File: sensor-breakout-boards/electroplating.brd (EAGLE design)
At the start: 25.4 x 25.4 mm, 4 parts, among them X1 Type-A Receptacle, X2 10-PIN-CONNECTOR

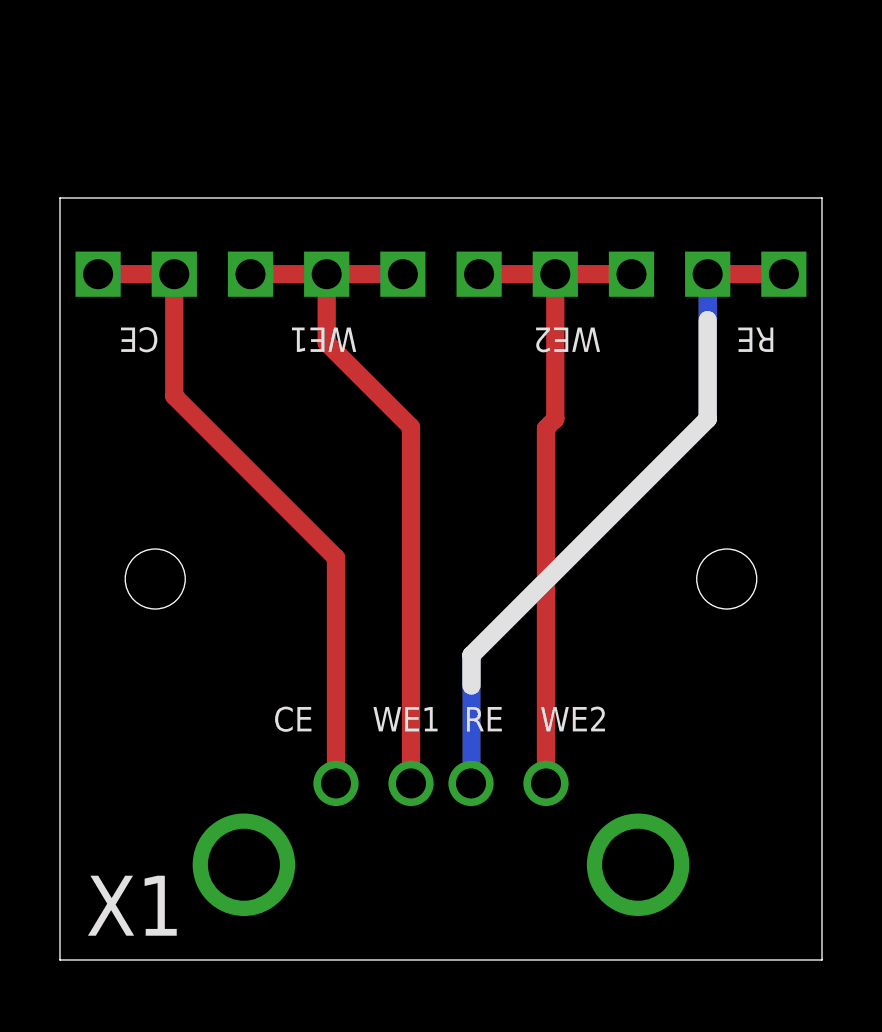
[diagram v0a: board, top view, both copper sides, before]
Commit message: made changes discussed at meeting
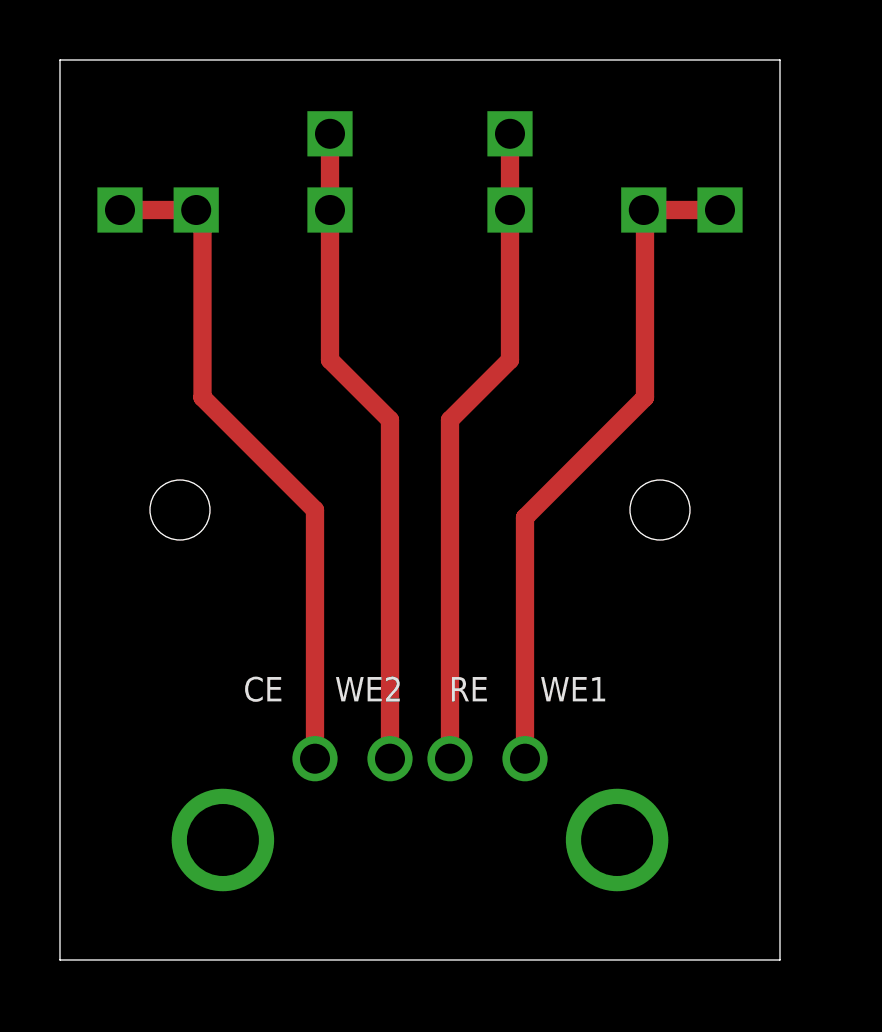
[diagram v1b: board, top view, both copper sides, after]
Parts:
- added X3, X4, X5: 2-PIN-CONNECTOR, sensor-breakout-boards:2-PIN-HEADER
- X2: value 10-PIN-CONNECTOR -> 2-PIN-CONNECTOR; device sensor-breakout-boards:10-PIN-HEADER -> sensor-breakout-boards:2-PIN-HEADER
- moved X2 10.9 mm to (2.00, 25.0)
- moved MOUNTING1 3.20 mm to (20.0, 15.0)
- moved MOUNTING2 2.44 mm to (4.00, 15.0)
- moved X1 1.08 mm to (12.0, 4.00)
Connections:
- net RE: now also X4.1, X4.2; no longer X2.10, X2.9
- net WE1: now also X1.4, X5.1, X5.2; no longer X1.2, X2.3, X2.4, X2.5
- net WE2: now also X1.2, X3.1, X3.2; no longer X1.4, X2.6, X2.7, X2.8
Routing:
- net RE: track 22.8 -> 21.7 mm
- net CE: track 21.7 -> 22.5 mm
- net WE1: track 23.2 -> 22.5 mm
- net WE2: track 22.2 -> 21.7 mm
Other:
- board size 25.4 x 25.4 mm -> 24 x 30 mm
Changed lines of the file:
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@@
 <setting verticaltext="up"/>
 </settings>
-<grid distance="0.01" unitdist="inch" unit="inch" style="lines" multiple="1" display="no" altdistance="0.025" altunitdist="inch" altunit="inch"/>
+<grid distance="0.25" unitdist="mm" unit="mm" style="lines" multiple="1" display="no" altdistance="0.025" altunitdist="inch" altunit="inch"/>
 <layers>
 <layer number="1" name="Top" color="4" fill="1" visible="yes" active="yes"/>
@@
 <board>
 <plain>
-<wire x1="0" y1="0" x2="25.4" y2="0" width="0" layer="20"/>
-<wire x1="25.4" y1="0" x2="25.4" y2="25.4" width="0" layer="20"/>
-<wire x1="25.4" y1="25.4" x2="0" y2="25.4" width="0" layer="20"/>
-<wire x1="0" y1="25.4" x2="0" y2="0" width="0" layer="20"/>
-<text x="7.112" y="7.62" size="0.8128" layer="21">CE</text>
-<text x="10.414" y="7.62" size="0.8128" layer="21">WE1</text>
-<text x="13.462" y="7.62" size="0.8128" layer="21">RE</text>
-<text x="16.002" y="7.62" size="0.8128" layer="21">WE2</text>
-<wire x1="13.716" y1="9.144" x2="13.716" y2="10.16" width="0.6096" layer="21"/>
-<wire x1="13.716" y1="10.16" x2="21.59" y2="18.034" width="0.6096" layer="21"/>
-<wire x1="21.59" y1="18.034" x2="21.59" y2="21.336" width="0.6096" layer="21"/>
-<text x="3.302" y="21.082" size="0.8128" layer="21" rot="SR180">CE</text>
-<text x="9.906" y="21.082" size="0.8128" layer="21" rot="SR180">WE1</text>
-<text x="18.034" y="21.082" size="0.8128" layer="21" rot="SR180">WE2</text>
-<text x="23.876" y="21.082" size="0.8128" layer="21" rot="SR180">RE</text>
+<wire x1="0" y1="0" x2="24" y2="0" width="0" layer="20"/>
+<wire x1="24" y1="0" x2="24" y2="30" width="0" layer="20"/>
+<wire x1="24" y1="30" x2="0" y2="30" width="0" layer="20"/>
+<wire x1="0" y1="30" x2="0" y2="0" width="0" layer="20"/>
+<text x="6.112" y="8.62" size="0.8128" layer="21">CE</text>
+<text x="9.164" y="8.62" size="0.8128" layer="21">WE2</text>
+<text x="12.962" y="8.62" size="0.8128" layer="21">RE</text>
+<text x="16.002" y="8.62" size="0.8128" layer="21">WE1</text>
 </plain>
 <attributes>
@@
 </autorouter>
 <elements>
-<element name="X1" library="sensor-breakout-boards" package="TE_CONNECTIVITY_292303-1" value="Type-A Receptacle" x="12.7" y="3.175" smashed="yes">
-<attribute name="NAME" x="0.858" y="0.809" size="2" layer="25" font="vector"/>
-</element>
-<element name="X2" library="sensor-breakout-boards" package="10-PIN-HEADER" value="10-PIN-CONNECTOR" x="12.7" y="22.86"/>
-<element name="MOUNTING1" library="sensor-breakout-boards" package="M2-MOUNTING-HOLE" value="M2-MOUNTING-HOLE" x="22.225" y="12.7"/>
-<element name="MOUNTING2" library="sensor-breakout-boards" package="M2-MOUNTING-HOLE" value="M2-MOUNTING-HOLE" x="3.175" y="12.7"/>
+<element name="X1" library="sensor-breakout-boards" package="TE_CONNECTIVITY_292303-1" value="Type-A Receptacle" x="12" y="4" smashed="yes"/>
+<element name="MOUNTING1" library="sensor-breakout-boards" package="M2-MOUNTING-HOLE" value="M2-MOUNTING-HOLE" x="20" y="15"/>
+<element name="MOUNTING2" library="sensor-breakout-boards" package="M2-MOUNTING-HOLE" value="M2-MOUNTING-HOLE" x="4" y="15"/>
+<element name="X2" library="sensor-breakout-boards" package="2-PIN-HEADER" value="2-PIN-CONNECTOR" x="2" y="25"/>
+<element name="X3" library="sensor-breakout-boards" package="2-PIN-HEADER" value="2-PIN-CONNECTOR" x="9" y="25" rot="R90"/>
+<element name="X4" library="sensor-breakout-boards" package="2-PIN-HEADER" value="2-PIN-CONNECTOR" x="15" y="25" rot="R90"/>
+<element name="X5" library="sensor-breakout-boards" package="2-PIN-HEADER" value="2-PIN-CONNECTOR" x="22" y="25" rot="R180"/>
 </elements>
 <signals>
 <signal name="CE">
+<contactref element="X1" pad="1"/>
+<contactref element="X2" pad="2"/>
 <contactref element="X2" pad="1"/>
-<contactref element="X2" pad="2"/>
-<contactref element="X1" pad="1"/>
-<wire x1="1.27" y1="22.86" x2="3.81" y2="22.86" width="0.6096" layer="1"/>
-<wire x1="3.81" y1="22.86" x2="3.81" y2="18.796" width="0.6096" layer="1"/>
-<wire x1="9.2" y1="5.885" x2="9.2" y2="13.406" width="0.6096" layer="1"/>
-<wire x1="9.2" y1="13.406" x2="3.81" y2="18.796" width="0.6096" layer="1"/>
+<wire x1="2" y1="25" x2="4.54" y2="25" width="0.6096" layer="1"/>
+<wire x1="8.5" y1="6.71" x2="8.5" y2="15" width="0.6096" layer="1"/>
+<wire x1="8.5" y1="15" x2="4.75" y2="18.75" width="0.6096" layer="1"/>
+<wire x1="4.75" y1="18.75" x2="4.75" y2="24.79" width="0.6096" layer="1"/>
+<wire x1="4.75" y1="24.79" x2="4.54" y2="25" width="0.6096" layer="1"/>
+</signal>
+<signal name="WE2">
+<contactref element="X1" pad="2"/>
+<contactref element="X3" pad="2"/>
+<contactref element="X3" pad="1"/>
+<wire x1="9" y1="27.54" x2="9" y2="25" width="0.6096" layer="1"/>
+<wire x1="11" y1="6.71" x2="11" y2="18" width="0.6096" layer="1"/>
+<wire x1="11" y1="18" x2="9" y2="20" width="0.6096" layer="1"/>
+<wire x1="9" y1="20" x2="9" y2="25" width="0.6096" layer="1"/>
 </signal>
 <signal name="WE1">
-<contactref element="X2" pad="3"/>
-<contactref element="X2" pad="4"/>
-<contactref element="X2" pad="5"/>
-<contactref element="X1" pad="2"/>
-<wire x1="6.35" y1="22.86" x2="8.89" y2="22.86" width="0.6096" layer="1"/>
-<wire x1="8.89" y1="22.86" x2="11.43" y2="22.86" width="0.6096" layer="1"/>
-<wire x1="11.7" y1="5.885" x2="11.7" y2="17.764" width="0.6096" layer="1"/>
-<wire x1="11.7" y1="17.764" x2="8.89" y2="20.574" width="0.6096" layer="1"/>
-<wire x1="8.89" y1="20.574" x2="8.89" y2="22.86" width="0.6096" layer="1"/>
-</signal>
-<signal name="WE2">
-<contactref element="X2" pad="6"/>
-<contactref element="X2" pad="7"/>
-<contactref element="X2" pad="8"/>
 <contactref element="X1" pad="4"/>
-<wire x1="13.97" y1="22.86" x2="16.51" y2="22.86" width="0.6096" layer="1"/>
-<wire x1="16.51" y1="22.86" x2="19.05" y2="22.86" width="0.6096" layer="1"/>
-<wire x1="16.2" y1="5.885" x2="16.2" y2="17.724" width="0.6096" layer="1"/>
-<wire x1="16.2" y1="17.724" x2="16.51" y2="18.034" width="0.6096" layer="1"/>
-<wire x1="16.51" y1="18.034" x2="16.51" y2="22.86" width="0.6096" layer="1"/>
+<contactref element="X5" pad="1"/>
+<contactref element="X5" pad="2"/>
+<wire x1="15.5" y1="6.71" x2="15.5" y2="14.75" width="0.6096" layer="1"/>
+<wire x1="15.5" y1="14.75" x2="19.5" y2="18.75" width="0.6096" layer="1"/>
+<wire x1="19.5" y1="18.75" x2="19.5" y2="24.96" width="0.6096" layer="1"/>
+<wire x1="19.5" y1="24.96" x2="19.46" y2="25" width="0.6096" layer="1"/>
+<wire x1="19.46" y1="25" x2="22" y2="25" width="0.6096" layer="1"/>
 </signal>
 <signal name="RE">
-<contactref element="X2" pad="9"/>
-<contactref element="X2" pad="10"/>
 <contactref element="X1" pad="3"/>
-<wire x1="21.59" y1="22.86" x2="24.13" y2="22.86" width="0.6096" layer="1"/>
-<wire x1="21.59" y1="22.86" x2="21.59" y2="18.034" width="0.6096" layer="16"/>
-<wire x1="21.59" y1="18.034" x2="13.716" y2="10.16" width="0.6096" layer="16"/>
-<wire x1="13.716" y1="10.16" x2="13.716" y2="5.901" width="0.6096" layer="16"/>
-<wire x1="13.716" y1="5.901" x2="13.7" y2="5.885" width="0.6096" layer="16"/>
+<contactref element="X4" pad="1"/>
+<contactref element="X4" pad="2"/>
+<wire x1="15" y1="27.54" x2="15" y2="25.5" width="0.6096" layer="1"/>
+<wire x1="15" y1="25.5" x2="15" y2="25" width="0.6096" layer="1"/>
+<wire x1="13" y1="6.71" x2="13" y2="18" width="0.6096" layer="1"/>
+<wire x1="13" y1="18" x2="15" y2="20" width="0.6096" layer="1"/>
+<wire x1="15" y1="20" x2="15" y2="25" width="0.6096" layer="1"/>
 </signal>
 </signals>
